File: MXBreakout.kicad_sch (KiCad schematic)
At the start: 17 parts, among them U1 Wii-MX, Y1 32.768kHz

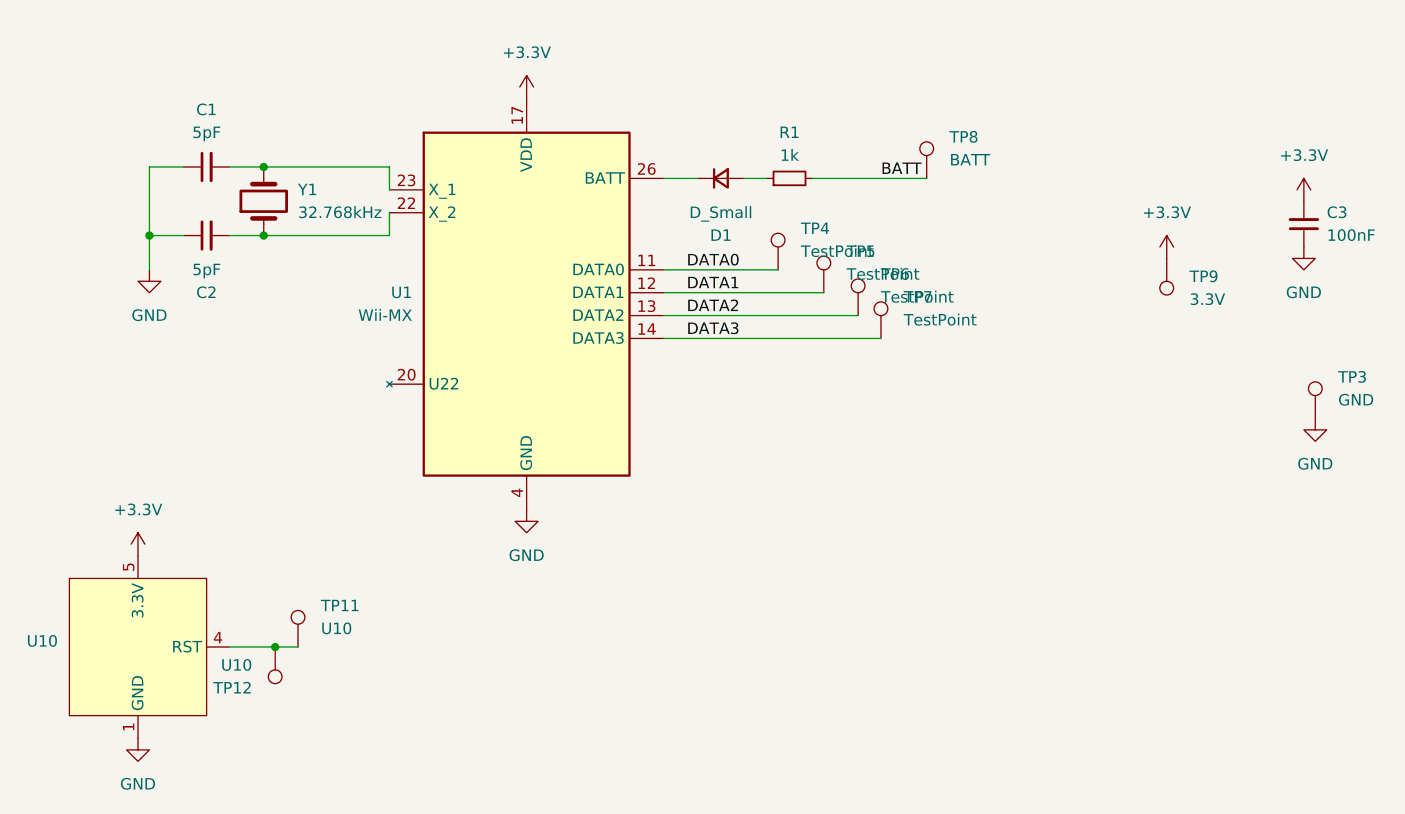
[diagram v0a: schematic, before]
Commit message: Minor cleanup
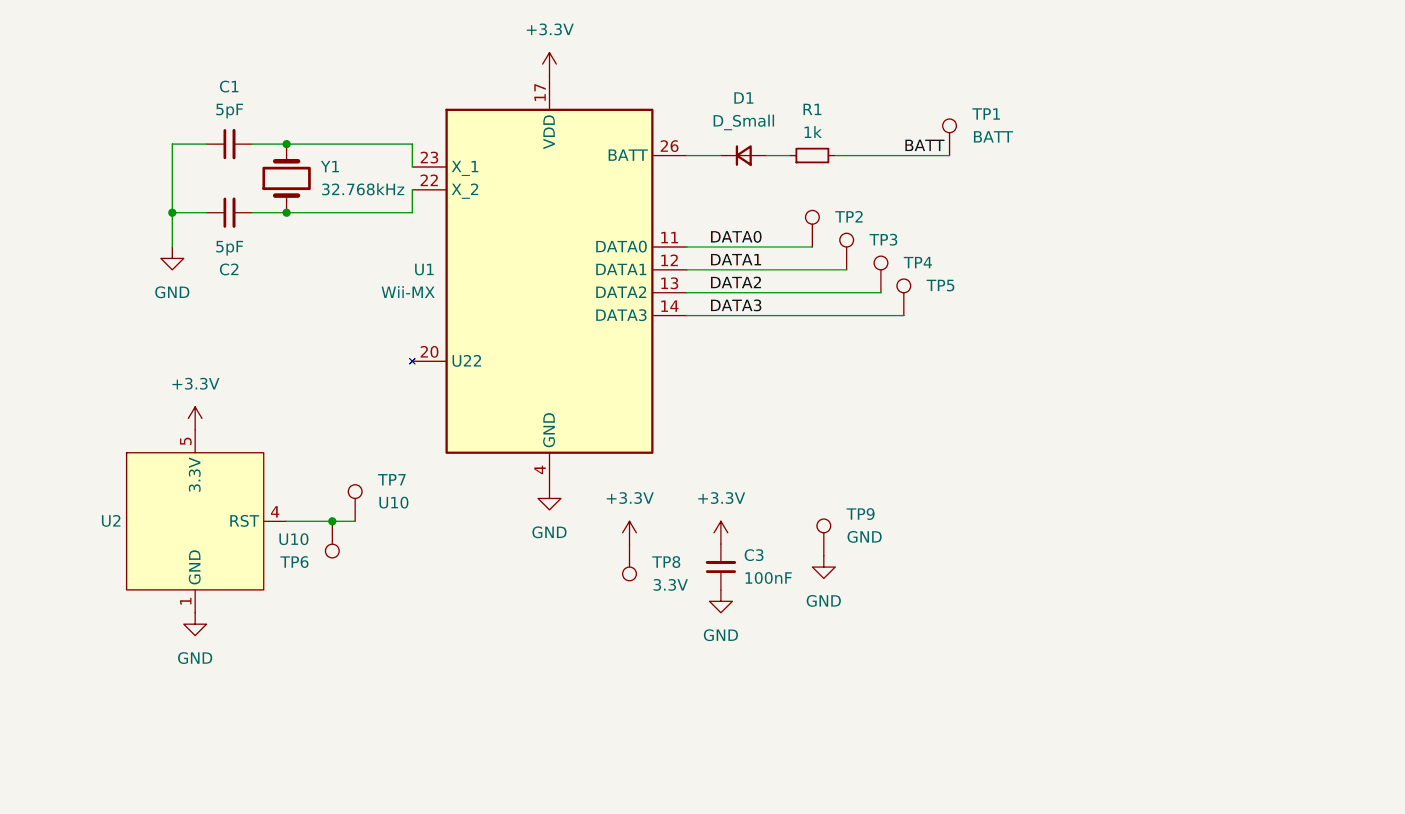
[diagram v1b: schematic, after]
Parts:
- removed TP11: U10, Wii:TestPoint_THTPad_D0.5mm_Drill0.35mm, symbol Connector:TestPoint
- removed TP12: U10, TestPoint:TestPoint_Pad_D1.0mm, symbol Connector:TestPoint
- removed U10: ~, Package_TO_SOT_SMD:SOT-23-5, symbol Wii:U10
- added TP1: BATT, TestPoint:TestPoint_Pad_D1.0mm, symbol Connector:TestPoint
- added TP2: DATA0, Wii:TestPoint_THTPad_D0.5mm_Drill0.35mm, symbol Connector:TestPoint
- added U2: ~, Package_TO_SOT_SMD:SOT-23-5, symbol Wii:U10
- TP3: value GND -> DATA1
- TP4: value TestPoint -> DATA2
- TP5: value TestPoint -> DATA3
- TP6: value TestPoint -> U10; footprint Wii:TestPoint_THTPad_D0.5mm_Drill0.35mm -> TestPoint:TestPoint_Pad_D1.0mm
- TP7: value TestPoint -> U10
- TP8: value BATT -> 3.3V
- TP9: value 3.3V -> GND; footprint TestPoint:TestPoint_Pad_D1.0mm -> Wii:TestPoint_THTPad_D0.5mm_Drill0.35mm
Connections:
- net +3.3V: now also TP8.1, U2.5 (3.3V); no longer TP9.1
- net BATT: now also TP1.1; no longer TP8.1
- net DATA0: now also TP2.1; no longer TP4.1
- net DATA1: now also TP3.1; no longer TP5.1
- net DATA2: now also TP4.1; no longer TP6.1
- net DATA3: now also TP5.1; no longer TP7.1
- net GND: now also TP9.1, U2.1 (GND), U2.2 (GND), U2.3 (GND); no longer TP3.1
- new net: TP6.1, TP7.1, U2.4 (RST)
